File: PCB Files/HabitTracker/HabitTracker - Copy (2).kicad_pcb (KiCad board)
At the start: 2 copper layers, 39 parts, among them U1 TLC5955DCA, U2 DCA0056F_N, U3 DCA0056F_N

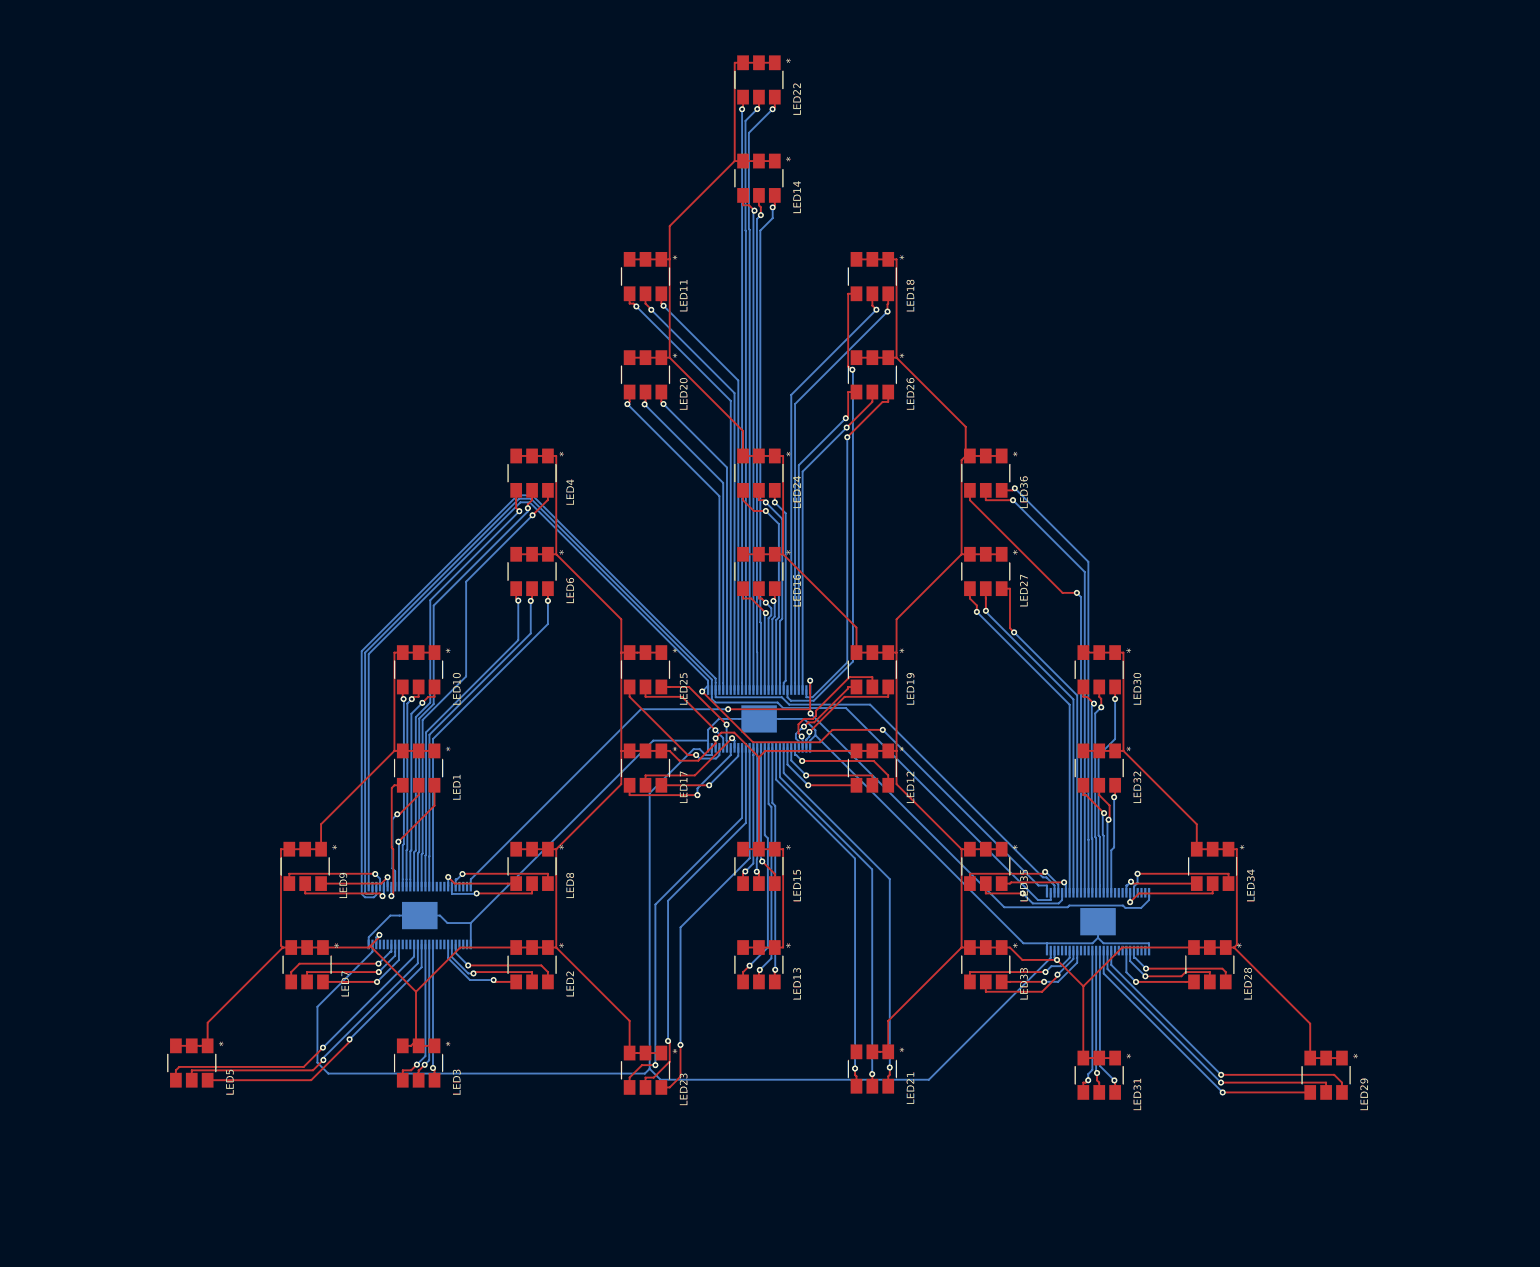
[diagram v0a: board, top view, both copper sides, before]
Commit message: Updated PCB
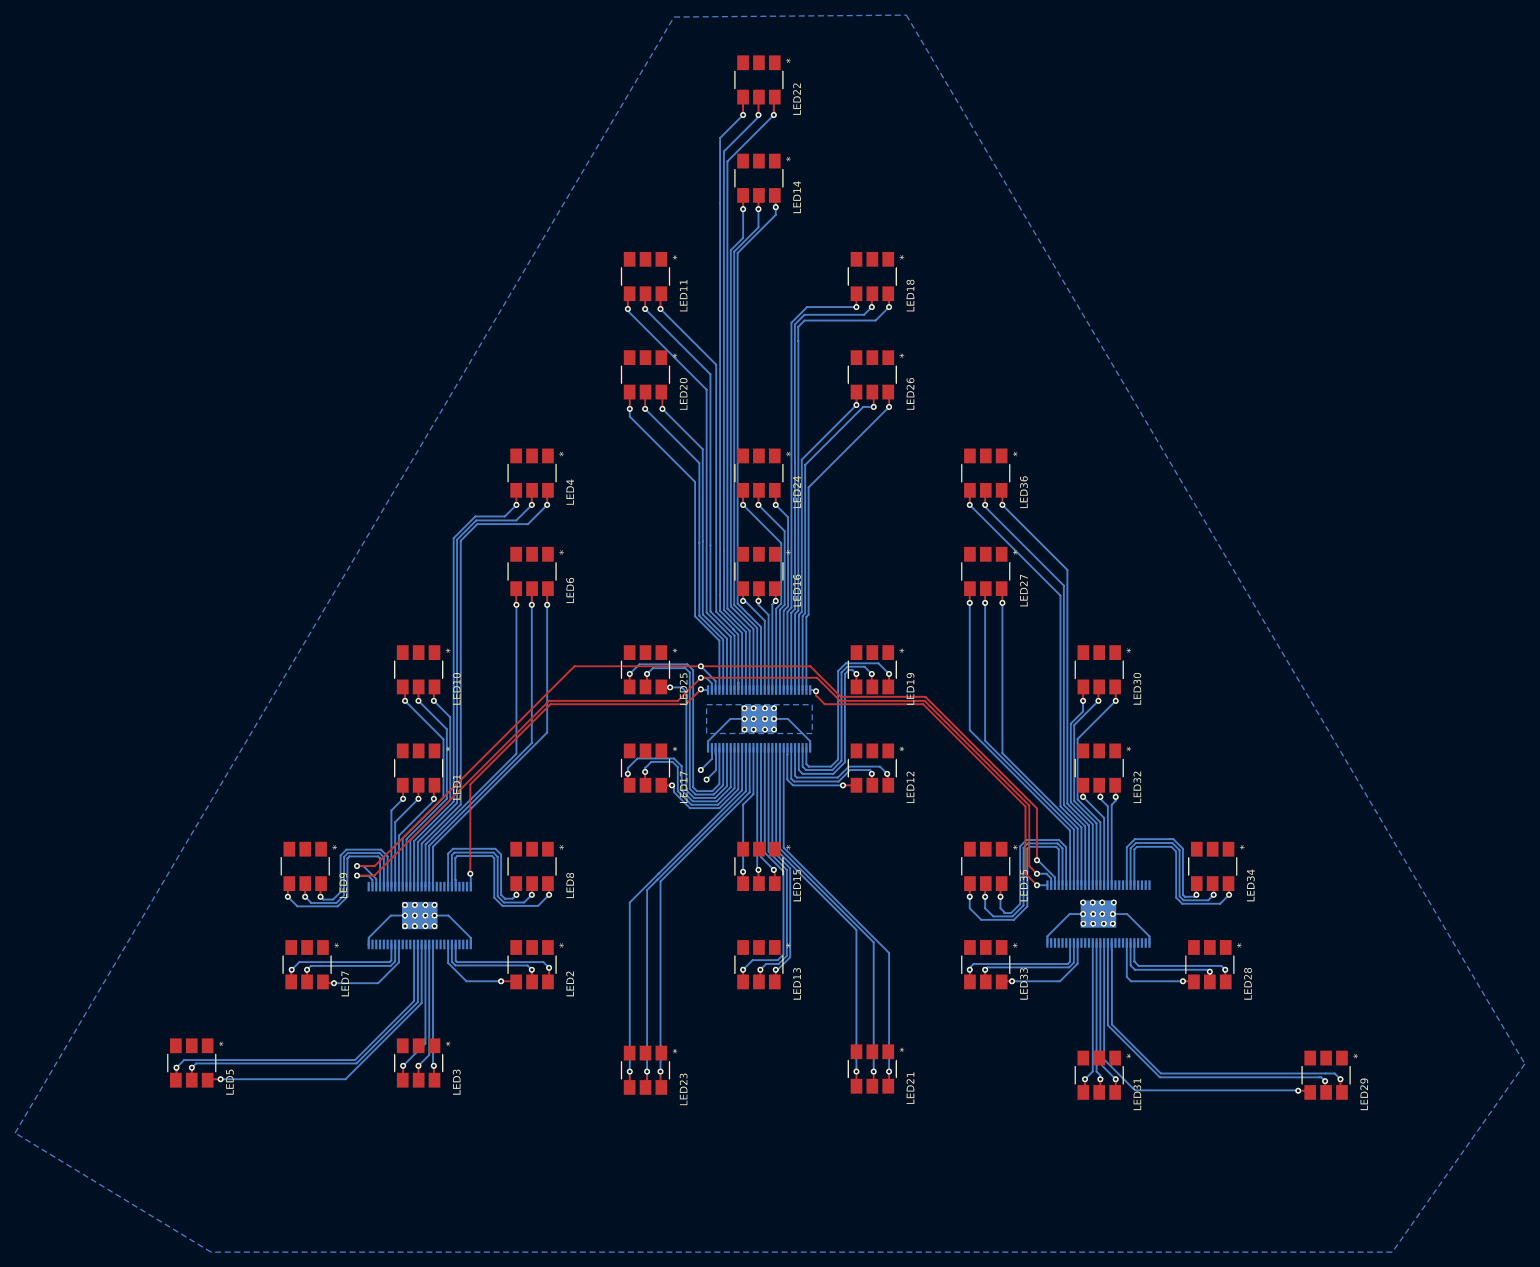
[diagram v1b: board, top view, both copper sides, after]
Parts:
- U2, U3: value DCA0056F_N -> TLC5955DCA
- moved U3 1.01 mm to (199.9, 130.3)
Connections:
- U2 pad 1: /SERIAL_IN -> /SERIAL_LINK1
- U2 pad 28: /SERIAL_LINK1 -> /SERIAL_LINK2
- U3 pad 1: /SERIAL_IN -> /SERIAL_LINK2
- U3 pad 28: /SERIAL_LINK1 -> /SERIAL_OUT
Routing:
- net +5V: track 741.5 -> 4.73 mm, vias 3 -> 1
- net /GS_CLOCK: track 173.1 -> 3.55 mm, vias 0 -> 1
- net /SERIAL_IN: track 154.5 -> 0.00 mm, vias 2 -> 0
- net GND: track 140.8 -> 47.3 mm, vias 0 -> 36
- net /SERIAL_LINK1: track 117.8 -> 50.2 mm, vias 3 -> 2
- net /SERIAL_LINK2: track 0.00 -> 47.6 mm, vias 0 -> 2
- net /SERIAL_CLOCK: track 157.3 -> 125.0 mm, vias 0 -> 3
- net /LATCH: track 159.4 -> 128.1 mm, vias 0 -> 3
- net Net-(LED25-Pad5): track 15.1 -> 33.6 mm
- net Net-(LED25-Pad4): track 17.7 -> 35.3 mm
- net Net-(LED35-Pad6): track 9.79 -> 26.2 mm
- net Net-(LED35-Pad5): track 13.1 -> 27.6 mm
- net Net-(LED25-Pad6): track 13.8 -> 28.1 mm
- net Net-(LED35-Pad4): track 14.9 -> 29.0 mm
- net Net-(LED19-Pad4): track 12.7 -> 25.2 mm
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- added copper zone on B.Cu, net GND
